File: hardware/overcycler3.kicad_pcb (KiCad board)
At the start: 2 copper layers, 208.3 x 152.4 mm, 279 parts, among them IC1 LM13700, IC2 LM13700, IC3 LM13700, P1 LPC_P1, P2 LPC_P2, P3 FT232, P4 PANEL, P5 SDCARD, P6 MIDI_IN, P7 FOOT_IN, P8 AC_IN, P9 AUDIO_OUT, Q1 BC547, SW1 RESET, U1 TLV1543, U10 MCP4922-E/P, U11 SSM2044, U12 MCP4922-E/P, U13 SSM2044, U14 MCP4922-E/P, U15 SSM2044, U16 MCP4922-E/P, U17 SSM2044, U18 MCP4922-E/P, U19 SSM2044, U2 74HC138, U20 MCP4922-E/P, U21 SSM2044, U3 LTC1660, U4 LTC1660, U5 TL074, U6 TL074, U7 LM1084IT-5.0/NOPB, U8 LM2990-5.0/NOPB, U9 LM1084IT-ADJ/NOPB

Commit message: hardware: beginning of overcycler 3 PCB
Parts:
- removed D6, D7: 1N5819, D3
- removed P3: FT232, SIL-6
- removed P4: PANEL, CONN40
- removed P5: SDCARD, SIL-7
- removed P6: MIDI_IN, SIL-2
- removed P7: FOOT_IN, SIL-2
- removed P8: AC_IN, bornier2
- removed P9: AUDIO_OUT, SIL-8
- removed R100, R105, R67, R68, R83, R85: 15k, R3-LARGE_PADS
- removed R101, R71: 6k8, R3-LARGE_PADS
- removed R102, R117, R54, R84: 820, R3-LARGE_PADS
- removed R118, R88: 390, R3-LARGE_PADS
- removed R119, R122, R50: 4k7, R3-LARGE_PADS
- removed R49, R51, R66: 22k, R3-LARGE_PADS
- removed RV2, RV3, RV4, RV5, RV6, RV7: 1k, RV2X1.5
- removed U20: MCP4922-E/P, DIP-14__300_ELL
- removed U21: SSM2044, DIP-16__300_ELL
- added C100: 470n, Capacitor_SMD:C_0805_2012Metric, F.Cu at (236.2, 123.9)
- added C101: 100u, Capacitor_Tantalum_SMD:CP_EIA-3528-21_Kemet-B, F.Cu at (247.9, 123.5)
- added C102: 22u, Capacitor_Tantalum_SMD:CP_EIA-3216-18_Kemet-A, F.Cu at (247.8, 139.9)
- added C103: 22u, Capacitor_Tantalum_SMD:CP_EIA-3216-18_Kemet-A, F.Cu at (247.8, 143.1)
- added C104: 470n, Capacitor_SMD:C_0805_2012Metric, F.Cu at (236.2, 147.3)
- added C105: 10n, Capacitor_SMD:C_1206_3216Metric, F.Cu at (242.1, 140.0)
- added C106: 10n, Capacitor_SMD:C_1206_3216Metric, F.Cu at (242.1, 143.3)
- added C107: 10n, Capacitor_SMD:C_1206_3216Metric, F.Cu at (242.1, 146.7)
- added C108: 820p, Capacitor_SMD:C_0603_1608Metric, F.Cu at (241.3, 149.6)
- added C109: 33u, Capacitor_Tantalum_SMD:CP_EIA-3216-18_Kemet-A, F.Cu at (247.8, 146.2)
- added C110: 470n, Capacitor_SMD:C_0805_2012Metric, F.Cu at (236.2, 150.3)
- added C111: 100u, Capacitor_Tantalum_SMD:CP_EIA-3528-21_Kemet-B, F.Cu at (247.9, 149.9)
- added C96: 10n, Capacitor_SMD:C_1206_3216Metric, F.Cu at (242.1, 117.0)
- added C97: 10n, Capacitor_SMD:C_1206_3216Metric, F.Cu at (242.1, 120.3)
- added C98: 820p, Capacitor_SMD:C_0603_1608Metric, F.Cu at (241.3, 123.2)
- added C99: 33u, Capacitor_Tantalum_SMD:CP_EIA-3216-18_Kemet-A, F.Cu at (247.8, 119.8)
- added FB1: FerriteBead, Inductor_SMD:L_0805_2012Metric, F.Cu at (25.4, 31.8)
- added J1: USB_B, Connector_USB:USB_B_Lumberg_2411_02_Horizontal, F.Cu at (37.2, 30.3)
- added J2: AudioJack3_Switch, Connector_Audio:Jack_6.35mm_Neutrik_NMJ6HFD2_Horizontal, F.Cu at (96.0, 37.4)
- added J3: DIN-5_180degree, DIN-5-180:DIN-5-180, F.Cu at (129.7, 29.8)
- added J4: AudioJack3_Switch, Connector_Audio:Jack_6.35mm_Neutrik_NMJ6HFD2_Horizontal, F.Cu at (169.7, 37.5)
- added J5: AudioJack3_Switch, Connector_Audio:Jack_6.35mm_Neutrik_NMJ6HFD2_Horizontal, F.Cu at (192.1, 37.5)
- added PS1: IA0505S-2W, JETEKPS:IA0505S-2W, F.Cu at (45.7, 55.9)
- added PS2: IB0503LSY-1WR1, JETEKPS:IB0503LSY, F.Cu at (38.1, 40.6)
- added R: 15k, Resistor_SMD:R_0805_2012Metric, F.Cu at (168.6, 132.7)
- added R: 15k, Resistor_SMD:R_0805_2012Metric, F.Cu at (228.2, 117.9)
- added R: 15k, Resistor_SMD:R_0805_2012Metric, F.Cu at (197.9, 135.7)
- added R: 15k, Resistor_SMD:R_0805_2012Metric, F.Cu at (168.6, 144.5)
- added R: 15k, Resistor_SMD:R_0805_2012Metric, F.Cu at (228.2, 106.1)
- added R: 15k, Resistor_SMD:R_0805_2012Metric, F.Cu at (197.9, 144.5)
- added R: 15k, Resistor_SMD:R_0805_2012Metric, F.Cu at (228.2, 129.6)
- added R: 15k, Resistor_SMD:R_0805_2012Metric, F.Cu at (228.2, 103.2)
- added R: 15k, Resistor_SMD:R_0805_2012Metric, F.Cu at (197.9, 132.7)
- added R: 15k, Resistor_SMD:R_0805_2012Metric, F.Cu at (228.2, 109.1)
- added R: 15k, Resistor_SMD:R_0805_2012Metric, F.Cu at (139.2, 144.5)
- added R: 15k, Resistor_SMD:R_0805_2012Metric, F.Cu at (228.2, 132.5)
- added R: 15k, Resistor_SMD:R_0805_2012Metric, F.Cu at (228.2, 144.3)
- added R: 15k, Resistor_SMD:R_0805_2012Metric, F.Cu at (109.8, 135.7)
- added R: 15k, Resistor_SMD:R_0805_2012Metric, F.Cu at (109.8, 132.7)
- added R: 15k, Resistor_SMD:R_0805_2012Metric, F.Cu at (168.6, 135.7)
- added R: 15k, Resistor_SMD:R_0805_2012Metric, F.Cu at (228.2, 135.5)
- added R: 15k, Resistor_SMD:R_0805_2012Metric, F.Cu at (139.2, 129.8)
- added R: 15k, Resistor_SMD:R_0805_2012Metric, F.Cu at (109.8, 144.5)
- added R: 15k, Resistor_SMD:R_0805_2012Metric, F.Cu at (197.9, 129.8)
- added R: 15k, Resistor_SMD:R_0805_2012Metric, F.Cu at (139.2, 132.7)
- added R: 15k, Resistor_SMD:R_0805_2012Metric, F.Cu at (139.2, 135.7)
- added R: 15k, Resistor_SMD:R_0805_2012Metric, F.Cu at (109.8, 129.8)
- added R: 15k, Resistor_SMD:R_0805_2012Metric, F.Cu at (168.6, 129.8)
- added R131: 820, Resistor_SMD:R_0805_2012Metric, F.Cu at (237.1, 109.1)
- added R132: 22k, Resistor_SMD:R_0805_2012Metric, F.Cu at (237.1, 112.0)
- added R133: 4k7, Resistor_SMD:R_0805_2012Metric, F.Cu at (237.1, 115.0)
- added R137: 6k8, Resistor_SMD:R_0805_2012Metric, F.Cu at (228.2, 138.4)
- added R138: 15k, Resistor_SMD:R_0805_2012Metric, F.Cu at (228.2, 141.4)
- added R140: 390, Resistor_SMD:R_0805_2012Metric, F.Cu at (232.7, 129.6)
- added R141: 820, Resistor_SMD:R_0805_2012Metric, F.Cu at (232.7, 132.5)
- added R142: 15k, Resistor_SMD:R_0805_2012Metric, F.Cu at (232.7, 135.5)
- added R143: 4k7, Resistor_SMD:R_0805_2012Metric, F.Cu at (232.7, 138.4)
- added R144: 10k, Resistor_SMD:R_0805_2012Metric, F.Cu at (232.7, 141.4)
- added R145: 470, Resistor_SMD:R_0805_2012Metric, F.Cu at (232.7, 144.3)
- added R146: 470, Resistor_SMD:R_0805_2012Metric, F.Cu at (237.1, 129.6)
- added R147: 4k7, Resistor_SMD:R_0805_2012Metric, F.Cu at (237.1, 132.5)
- added R148: 820, Resistor_SMD:R_0805_2012Metric, F.Cu at (237.1, 135.5)
- added R149: 22k, Resistor_SMD:R_0805_2012Metric, F.Cu at (237.1, 138.4)
- added R150: 4k7, Resistor_SMD:R_0805_2012Metric, F.Cu at (237.1, 141.4)
- added SW2: POWER, SPUN192600:SPUN192600, F.Cu at (53.3, 30.3)
- added Y1: 12MHz, Crystal:Crystal_SMD_HC49-SD, F.Cu at (53.3, 82.5)
- C1: value 10u -> 22p; footprint C1V5 -> Capacitor_SMD:C_0805_2012Metric
- C10, C11, C37, C38, C39, C46, C47, C8: value 10n -> 100n; footprint C2 -> Capacitor_SMD:C_0805_2012Metric
- C12, C14, C15, C16, C17, C18, C19, C20, C26, C27, C30, C6, C7, C90, C94: footprint C2 -> Capacitor_SMD:C_0805_2012Metric
- C13: value 100n -> 470u; footprint C2 -> Capacitor_Tantalum_SMD:CP_EIA-7343-43_Kemet-X
- C2, C3, C4: value 100n -> 10n; footprint C2 -> Capacitor_SMD:C_0805_2012Metric
- C21, C22: value 100n -> 10u; footprint C2 -> Capacitor_Tantalum_SMD:CP_EIA-3216-18_Kemet-A
- C23, C42: value 100u -> 100n; footprint C1.5V8V -> Capacitor_SMD:C_0805_2012Metric
- C24, C25: value 10000u 16v -> 100n; footprint Elko_vert_DM16_RM7-5_CopperClear -> Capacitor_SMD:C_0805_2012Metric
- C28, C29: value 10u -> 100n; footprint C1V5 -> Capacitor_SMD:C_0805_2012Metric
- C31: value 100p -> 10u; footprint C2 -> Capacitor_Tantalum_SMD:CP_EIA-3216-18_Kemet-A
- C32: value 100p -> 100n; footprint C2 -> Capacitor_SMD:C_0805_2012Metric
- C33: value 10u -> 100u; footprint C1V5 -> Capacitor_Tantalum_SMD:CP_EIA-3528-21_Kemet-B
- C34, C35, C43, C44: value 22u -> 100n; footprint C1V7 -> Capacitor_SMD:C_0805_2012Metric
- C36, C81: value 820p -> 100u; footprint B32520-3 -> Capacitor_Tantalum_SMD:CP_EIA-3528-21_Kemet-B
- C40, C49: value 33u -> 100n; footprint C1.5V8V -> Capacitor_SMD:C_0805_2012Metric
- C41: value 470n -> 100n; footprint C2 -> Capacitor_SMD:C_0805_2012Metric
- C45: value 820p -> 100n; footprint B32520-3 -> Capacitor_SMD:C_0805_2012Metric
- C48: value 10n -> 100u; footprint C2 -> Capacitor_Tantalum_SMD:CP_EIA-3528-21_Kemet-B
- C5: value 100u -> 10n; footprint C1.5V8V -> Capacitor_SMD:C_0805_2012Metric
- C50: value 470n -> 100p; footprint C2 -> Capacitor_SMD:C_0805_2012Metric
- C51: value 100u -> 100p; footprint C1.5V8V -> Capacitor_SMD:C_0805_2012Metric
- C52, C53, C62: footprint C1V7 -> Capacitor_Tantalum_SMD:CP_EIA-3216-18_Kemet-A
- C54: value 820p -> 470n; footprint B32520-3 -> Capacitor_SMD:C_0805_2012Metric
- C55, C56, C57, C65, C66, C75: footprint C2 -> Capacitor_SMD:C_1206_3216Metric
- C58: value 33u -> 820p; footprint C1.5V8V -> Capacitor_SMD:C_0603_1608Metric
- C59, C89: value 470n -> 33u; footprint C2 -> Capacitor_Tantalum_SMD:CP_EIA-3216-18_Kemet-A
- C60: value 100u -> 470n; footprint C1.5V8V -> Capacitor_SMD:C_0805_2012Metric
- C61, C71: value 22u -> 100u; footprint C1V7 -> Capacitor_Tantalum_SMD:CP_EIA-3528-21_Kemet-B
- C63, C72: value 820p -> 22u; footprint B32520-3 -> Capacitor_Tantalum_SMD:CP_EIA-3216-18_Kemet-A
- C64, C74, C84: value 10n -> 470n; footprint C2 -> Capacitor_SMD:C_0805_2012Metric
- C67, C76, C85: value 33u -> 10n; footprint C1.5V8V -> Capacitor_SMD:C_1206_3216Metric
- C68: value 470n -> 820p; footprint C2 -> Capacitor_SMD:C_0603_1608Metric
- C69: value 100u -> 33u; footprint C1.5V8V -> Capacitor_Tantalum_SMD:CP_EIA-3216-18_Kemet-A
- C70, C80: value 22u -> 470n; footprint C1V7 -> Capacitor_SMD:C_0805_2012Metric
- C73, C82, C83: value 10n -> 22u; footprint C2 -> Capacitor_Tantalum_SMD:CP_EIA-3216-18_Kemet-A
- C77, C86: value 470n -> 10n; footprint C2 -> Capacitor_SMD:C_1206_3216Metric
- C78: value 100u -> 820p; footprint C1.5V8V -> Capacitor_SMD:C_0603_1608Metric
- C79: value 22u -> 33u; footprint C1V7 -> Capacitor_Tantalum_SMD:CP_EIA-3216-18_Kemet-A
- C87, C95: value 100u -> 10n; footprint C1.5V8V -> Capacitor_SMD:C_1206_3216Metric
- C88: value 2u2 -> 820p; footprint C1V5 -> Capacitor_SMD:C_0603_1608Metric
- C9: value 10n -> 22p; footprint C2 -> Capacitor_SMD:C_0805_2012Metric
- C91: value 470n -> 100u; footprint C2 -> Capacitor_Tantalum_SMD:CP_EIA-3528-21_Kemet-B
- C92, C93: value 470n -> 22u; footprint C2 -> Capacitor_Tantalum_SMD:CP_EIA-3216-18_Kemet-A
- D1: value 1N5819 -> 1N4148; footprint D3 -> Diode_SMD:D_SOD-123
- D2, D3, D4, D5: footprint D3 -> Diode_SMD:D_SOD-123
- IC1, IC2, IC3: footprint DIP-16__300_ELL -> Package_SO:SO-16_3.9x9.9mm_P1.27mm
- OC1: footprint optocoupler-DIL08 -> Package_DIP:DIP-8_W7.62mm
- P1: value LPC_P1 -> FT232; footprint SIL-33 -> Connector_PinSocket_2.54mm:PinSocket_1x06_P2.54mm_Vertical
- P2: value LPC_P2 -> PANEL; footprint SIL-33 -> Connector_IDC:IDC-Header_2x20_P2.54mm_Vertical
- Q1: value BC547 -> 2SC945; footprint TO92 -> Package_TO_SOT_SMD:SOT-23
- R1: value 270 -> 1k; footprint R3-LARGE_PADS -> Resistor_SMD:R_0805_2012Metric
- R10: value 1k -> 27k; footprint R3-LARGE_PADS -> Resistor_SMD:R_0805_2012Metric
- R103: value 390 -> 6k8; footprint R3-LARGE_PADS -> Resistor_SMD:R_0805_2012Metric
- R104, R125, R44, R74: value 4k7 -> 15k; footprint R3-LARGE_PADS -> Resistor_SMD:R_0805_2012Metric
- R106: value 10k -> 390; footprint R3-LARGE_PADS -> Resistor_SMD:R_0805_2012Metric
- R107, R80: value 4k7 -> 820; footprint R3-LARGE_PADS -> Resistor_SMD:R_0805_2012Metric
- R108, R57, R87: value 820 -> 15k; footprint R3-LARGE_PADS -> Resistor_SMD:R_0805_2012Metric
- R109, R79, R96: value 22k -> 4k7; footprint R3-LARGE_PADS -> Resistor_SMD:R_0805_2012Metric
- R11: value 10k -> 1k; footprint R3-LARGE_PADS -> Resistor_SMD:R_0805_2012Metric
- R110, R59, R7: value 4k7 -> 10k; footprint R3-LARGE_PADS -> Resistor_SMD:R_0805_2012Metric
- R111, R94: value 22k -> 470; footprint R3-LARGE_PADS -> Resistor_SMD:R_0805_2012Metric
- R112, R60: value 15k -> 470; footprint R3-LARGE_PADS -> Resistor_SMD:R_0805_2012Metric
- R113, R75, R82: value 15k -> 4k7; footprint R3-LARGE_PADS -> Resistor_SMD:R_0805_2012Metric
- R114, R12, R14, R28, R53, R62, R63, R64, R65, R70, R76, R81, R86, R92: footprint R3-LARGE_PADS -> Resistor_SMD:R_0805_2012Metric
- R115, R98: value 15k -> 22k; footprint R3-LARGE_PADS -> Resistor_SMD:R_0805_2012Metric
- R116: value 6k8 -> 4k7; footprint R3-LARGE_PADS -> Resistor_SMD:R_0805_2012Metric
- R120, R52: value 15k -> 6k8; footprint R3-LARGE_PADS -> Resistor_SMD:R_0805_2012Metric
- R121, R91: value 10k -> 15k; footprint R3-LARGE_PADS -> Resistor_SMD:R_0805_2012Metric
- R123, R72: value 820 -> 390; footprint R3-LARGE_PADS -> Resistor_SMD:R_0805_2012Metric
- R124: value 22k -> 820; footprint R3-LARGE_PADS -> Resistor_SMD:R_0805_2012Metric
- R126: value 220 -> 4k7; footprint R3-LARGE_PADS -> Resistor_SMD:R_0805_2012Metric
- R127: value 120 -> 10k; footprint R3-LARGE_PADS -> Resistor_SMD:R_0805_2012Metric
- R128, R129, R61: value 10k -> 470; footprint R3-LARGE_PADS -> Resistor_SMD:R_0805_2012Metric
- R13: value 100k -> 10k; footprint R3-LARGE_PADS -> Resistor_SMD:R_0805_2012Metric
- R130: value 1k -> 4k7; footprint R3-LARGE_PADS -> Resistor_SMD:R_0805_2012Metric
- R15: value 470 -> 100k; footprint R3-LARGE_PADS -> Resistor_SMD:R_0805_2012Metric
- R16: value 3M3 -> 4k7; footprint R3-LARGE_PADS -> Resistor_SMD:R_0805_2012Metric
- R17: value 470 -> 10k; footprint R3-LARGE_PADS -> Resistor_SMD:R_0805_2012Metric
- R18, R77, R95: value 4k7 -> 470; footprint R3-LARGE_PADS -> Resistor_SMD:R_0805_2012Metric
- R19: value 100k -> 3M3; footprint R3-LARGE_PADS -> Resistor_SMD:R_0805_2012Metric
- R2: value 4k7 -> 33; footprint R3-LARGE_PADS -> Resistor_SMD:R_0805_2012Metric
- R20: value 33k -> 470; footprint R3-LARGE_PADS -> Resistor_SMD:R_0805_2012Metric
- R21: value 47k -> 270; footprint R3-LARGE_PADS -> Resistor_SMD:R_0805_2012Metric
- R22: value 150k -> 4k7; footprint R3-LARGE_PADS -> Resistor_SMD:R_0805_2012Metric
- R23: value 56k -> 4k7; footprint R3-LARGE_PADS -> Resistor_SMD:R_0805_2012Metric
- R24: value 68k -> 100k; footprint R3-LARGE_PADS -> Resistor_SMD:R_0805_2012Metric
- R25: value 68k -> 1k; footprint R3-LARGE_PADS -> Resistor_SMD:R_0805_2012Metric
- R26: value 56k -> 220; footprint R3-LARGE_PADS -> Resistor_SMD:R_0805_2012Metric
- R27: value 150k -> 33k; footprint R3-LARGE_PADS -> Resistor_SMD:R_0805_2012Metric
- R29: value 33k -> 120k; footprint R3-LARGE_PADS -> Resistor_SMD:R_0805_2012Metric
- R3: value 220 -> 10k; footprint R3-LARGE_PADS -> Resistor_SMD:R_0805_2012Metric
- R30: value 15k -> 56k; footprint R3-LARGE_PADS -> Resistor_SMD:R_0805_2012Metric
- R31: value 15k -> 82k; footprint R3-LARGE_PADS -> Resistor_SMD:R_0805_2012Metric
- R32: value 47k -> 82k; footprint R3-LARGE_PADS -> Resistor_SMD:R_0805_2012Metric
- R33: value 47k -> 56k; footprint R3-LARGE_PADS -> Resistor_SMD:R_0805_2012Metric
- R34: value 1k -> 120k; footprint R3-LARGE_PADS -> Resistor_SMD:R_0805_2012Metric
- R35: value 1k -> 47k; footprint R3-LARGE_PADS -> Resistor_SMD:R_0805_2012Metric
- R36: value 22k -> 33k; footprint R3-LARGE_PADS -> Resistor_SMD:R_0805_2012Metric
- R37, R40: value 15k -> 1k; footprint R3-LARGE_PADS -> Resistor_SMD:R_0805_2012Metric
- R38: value 15k -> 2k2; footprint R3-LARGE_PADS -> Resistor_SMD:R_0805_2012Metric
- R39: value 820 -> 2k2; footprint R3-LARGE_PADS -> Resistor_SMD:R_0805_2012Metric
- R4: value 1k -> 33; footprint R3-LARGE_PADS -> Resistor_SMD:R_0805_2012Metric
- R41: value 6k8 -> 1k; footprint R3-LARGE_PADS -> Resistor_SMD:R_0805_2012Metric
- R42, R99: value 820 -> 4k7; footprint R3-LARGE_PADS -> Resistor_SMD:R_0805_2012Metric
- R43: value 390 -> 15k; footprint R3-LARGE_PADS -> Resistor_SMD:R_0805_2012Metric
- R45: value 15k -> 47k; footprint R3-LARGE_PADS -> Resistor_SMD:R_0805_2012Metric
- R46: value 10k -> 47k; footprint R3-LARGE_PADS -> Resistor_SMD:R_0805_2012Metric
- R47: value 4k7 -> 330; footprint R3-LARGE_PADS -> Resistor_SMD:R_0805_2012Metric
- R48: value 820 -> 330; footprint R3-LARGE_PADS -> Resistor_SMD:R_0805_2012Metric
- R5: value 10k -> 1k5; footprint R3-LARGE_PADS -> Resistor_SMD:R_0805_2012Metric
- R55: value 15k -> 390; footprint R3-LARGE_PADS -> Resistor_SMD:R_0805_2012Metric
- R56: value 6k8 -> 820; footprint R3-LARGE_PADS -> Resistor_SMD:R_0805_2012Metric
- R58: value 390 -> 4k7; footprint R3-LARGE_PADS -> Resistor_SMD:R_0805_2012Metric
- R6: value 470k -> 1k; footprint R3-LARGE_PADS -> Resistor_SMD:R_0805_2012Metric
- R69: value 820 -> 6k8; footprint R3-LARGE_PADS -> Resistor_SMD:R_0805_2012Metric
- R73: value 390 -> 820; footprint R3-LARGE_PADS -> Resistor_SMD:R_0805_2012Metric
- R78: value 820 -> 470; footprint R3-LARGE_PADS -> Resistor_SMD:R_0805_2012Metric
- R8: value 1M -> 470k; footprint R3-LARGE_PADS -> Resistor_SMD:R_0805_2012Metric
- R89: value 4k7 -> 390; footprint R3-LARGE_PADS -> Resistor_SMD:R_0805_2012Metric
- R9: value 27k -> 1M; footprint R3-LARGE_PADS -> Resistor_SMD:R_0805_2012Metric
- R90, R97: value 15k -> 820; footprint R3-LARGE_PADS -> Resistor_SMD:R_0805_2012Metric
- R93: value 820 -> 10k; footprint R3-LARGE_PADS -> Resistor_SMD:R_0805_2012Metric
- RV1: value 10k -> 47k; footprint RV2X1.5 -> Potentiometer_THT:Potentiometer_Alps_RK163_Dual_Horizontal
- SW1: footprint SW_PUSH_SMALL -> Button_Switch_THT:SW_PUSH_6mm
- U1: value TLV1543 -> XT26G02ELGIGA; footprint DIP-20__300_ELL -> Package_LGA:LGA-8_8x6mm_P1.27mm
- U10, U12, U14, U16, U18: value MCP4922-E/P -> MCP4922-ESL; footprint DIP-14__300_ELL -> Package_SO:SO-14_3.9x8.65mm_P1.27mm
- U11, U13, U15, U17, U19: value SSM2044 -> SSI2144; footprint DIP-16__300_ELL -> Package_SO:SSOP-16_3.9x4.9mm_P0.635mm
- U2: value 74HC138 -> TL074; footprint DIP-16__300_ELL -> Package_SO:SO-14_3.9x8.65mm_P1.27mm
- U3: value LTC1660 -> LPC1778FBD144; footprint DIP-16__300_ELL -> Package_QFP:LQFP-144_20x20mm_P0.5mm
- U4: value LTC1660 -> TLV1543; footprint DIP-16__300_ELL -> Package_SO:SOIC-20W_7.5x12.8mm_P1.27mm
- U5: value TL074 -> 74HC138; footprint DIP-14__300_ELL -> Package_SO:SO-16_3.9x9.9mm_P1.27mm
- U6: footprint DIP-14__300_ELL -> Package_SO:SO-14_3.9x8.65mm_P1.27mm
- U7: value LM1084IT-5.0/NOPB -> AD5674R; footprint TO220_VERT_FIXED -> Package_DFN_QFN:QFN-28-1EP_4x4mm_P0.4mm_EP2.6x2.6mm; moved to F.Cu
- U8: value LM2990-5.0/NOPB -> MCP4922-ESL; footprint TO220_VERT_FIXED -> Package_SO:SO-14_3.9x8.65mm_P1.27mm; moved to F.Cu
- U9: value LM1084IT-ADJ/NOPB -> SSI2144; footprint TO220_VERT_FIXED -> Package_SO:SSOP-16_3.9x4.9mm_P0.635mm; moved to F.Cu
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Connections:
- C1 pad 1: /DAC_VREF -> /XTAL1
- C11 pad 1: GND -> +5V
- C11 pad 2: -5V -> GND
- C13 pad 1: +5V -> Net-(PS1-+Vin)
- C13 pad 2: GND -> Net-(J1-GND)
- C18 pad 1: +5V -> +3.3V
- C19 pad 1: +5V -> +3.3V
- C2 pad 1: /DAC_VREF -> +5V
- C21 pad 1: +3.3V -> +5V
- C22 pad 1: +3.3V -> GND
- C22 pad 2: GND -> -5V
- C23 pad 1: N-0000012 -> +3.3V
- C23 pad 2: NOISE -> GND
- C24 pad 1: /UNR+ -> +3.3V
- C25 pad 1: GND -> +3.3V
- C25 pad 2: /UNR- -> GND
- C26 pad 1: /UNR+ -> +3.3V
- C27 pad 1: GND -> +3.3V
- C27 pad 2: /UNR- -> GND
- C28 pad 1: +5V -> +3.3V
- C29 pad 1: GND -> +3.3V
- C29 pad 2: -5V -> GND
- C3 pad 1: /FOOT_IN -> GND
- C3 pad 2: GND -> -5V
- C30 pad 1: +5V -> +3.3V
- C31 pad 1: N-0000073 -> +3.3V
- C31 pad 2: N-0000072 -> GND
- C32 pad 1: N-0000074 -> +3.3V
- C32 pad 2: N-0000071 -> GND
- C33 pad 1: +3.3V -> GND
- C33 pad 2: GND -> Net-(Q1-B)
- C34 pad 1: N-00000160 -> +3.3V
- C34 pad 2: N-00000163 -> GND
- C35 pad 1: N-00000161 -> Net-(Q1-E)
- C35 pad 2: N-00000162 -> Net-(U2A-+)
- C36 pad 1: N-00000164 -> Net-(C36-Pad1)
- C36 pad 2: N-00000179 -> GND
- C37 pad 1: N-00000180 -> /FOOT_IN
- C37 pad 2: N-00000166 -> GND
- C38 pad 1: N-00000170 -> /P_9
- C38 pad 2: N-00000169 -> GND
- C39 pad 1: N-00000167 -> /P_8
- C39 pad 2: N-00000171 -> GND
- C4 pad 1: N-000005 -> +5V
- C4 pad 2: N-0000017 -> GND
- C40 pad 1: N-00000172 -> /P_7
- C40 pad 2: N-00000178 -> GND
- C41 pad 1: -5V -> /P_6
- C41 pad 2: N-00000174 -> GND
- C42 pad 1: /Voice #0/OUT -> /P_5
- C42 pad 2: N-00000177 -> GND
- C43 pad 1: N-00000184 -> /P_0
- C43 pad 2: N-00000187 -> GND
- C44 pad 1: N-00000185 -> /P_1
- C44 pad 2: N-00000186 -> GND
- C45 pad 1: N-00000188 -> /P_2
- C45 pad 2: N-00000203 -> GND
- C46 pad 1: N-00000204 -> /P_3
- C46 pad 2: N-00000190 -> GND
- C47 pad 1: N-00000193 -> /P_4
- C47 pad 2: N-00000192 -> GND
- C48 pad 1: N-00000191 -> Net-(C48-Pad1)
- C48 pad 2: N-00000194 -> NOISE
- C49 pad 1: N-00000196 -> Net-(U4-REF+)
- C49 pad 2: N-00000202 -> GND
- C5 pad 1: N-0000020 -> GND
- C5 pad 2: GND -> -5V
- C50 pad 1: -5V -> Net-(U6B--)
- C50 pad 2: N-00000198 -> Net-(C50-Pad2)
- C51 pad 1: /Voice #1/OUT -> Net-(U6C--)
- C51 pad 2: N-00000201 -> Net-(C51-Pad2)
- C52 pad 1: N-00000209 -> Net-(U8-VoutA)
- C53 pad 1: N-00000210 -> Net-(U8-VoutB)
- C54 pad 1: N-00000213 -> GND
- C54 pad 2: N-00000227 -> Net-(U9-FREQ_CTRL)
- C55 pad 1: N-00000228 -> Net-(U9-C1B)
- C55 pad 2: N-00000215 -> Net-(U9-C1A)
- C56 pad 1: N-00000216 -> Net-(U9-C2B)
- C56 pad 2: N-00000219 -> Net-(U9-C2A)
- C57 pad 1: N-00000208 -> Net-(U9-C3A)
- C57 pad 2: N-00000217 -> Net-(U9-C3B)
- C58 pad 1: N-00000220 -> Net-(U9-C4A)
- C58 pad 2: N-00000226 -> Net-(U9-C4B)
- C59 pad 1: -5V -> Net-(U9-OUT)
- C59 pad 2: N-00000222 -> Net-(C59-Pad2)
- C60 pad 1: /Voice #2/OUT -> -5V
- C60 pad 2: N-00000225 -> Net-(IC1A-Iabc)
- C61 pad 1: N-00000233 -> /OUT_V0
- C61 pad 2: N-00000236 -> Net-(IC1A-buffer_out)
- C62 pad 1: N-00000234 -> Net-(U10-VoutA)
- C63 pad 1: N-00000237 -> Net-(U10-VoutB)
- C63 pad 2: N-00000251 -> Net-(C63-Pad2)
- C64 pad 1: N-00000252 -> GND
- C64 pad 2: N-00000239 -> Net-(U11-FREQ_CTRL)
- C65 pad 1: N-00000240 -> Net-(U11-C1B)
- C65 pad 2: N-00000238 -> Net-(U11-C1A)
- C66 pad 1: N-00000242 -> Net-(U11-C2B)
- C66 pad 2: N-00000241 -> Net-(U11-C2A)
- C67 pad 1: N-00000244 -> Net-(U11-C3A)
- C67 pad 2: N-00000250 -> Net-(U11-C3B)
- C68 pad 1: -5V -> Net-(U11-C4A)
- C68 pad 2: N-00000246 -> Net-(U11-C4B)
- C69 pad 1: /Voice #3/OUT -> Net-(U11-OUT)
- C69 pad 2: N-00000249 -> Net-(C69-Pad2)
- C70 pad 1: N-00000257 -> -5V
- C70 pad 2: N-00000260 -> Net-(IC2B-Iabc)
- C71 pad 1: N-00000258 -> /OUT_V3
- C71 pad 2: N-00000259 -> Net-(IC2B-buffer_out)
- C72 pad 1: N-00000261 -> Net-(U12-VoutA)
- C72 pad 2: N-00000275 -> Net-(C72-Pad2)
- C73 pad 1: N-00000276 -> Net-(U12-VoutB)
- C73 pad 2: N-00000264 -> Net-(C73-Pad2)
- C74 pad 1: N-00000265 -> GND
- C74 pad 2: N-00000256 -> Net-(U13-FREQ_CTRL)
- C75 pad 1: N-00000263 -> Net-(U13-C1B)
- C75 pad 2: N-00000266 -> Net-(U13-C1A)
- C76 pad 1: N-00000268 -> Net-(U13-C2B)
- C76 pad 2: N-00000274 -> Net-(U13-C2A)
- C77 pad 1: -5V -> Net-(U13-C3A)
- C77 pad 2: N-00000270 -> Net-(U13-C3B)
- C78 pad 1: /Voice #4/OUT -> Net-(U13-C4A)
- C78 pad 2: N-00000273 -> Net-(U13-C4B)
- C79 pad 1: N-00000280 -> Net-(U13-OUT)
- C79 pad 2: N-00000283 -> Net-(C79-Pad2)
- C8 pad 1: +5V -> /RESET
- C80 pad 1: N-00000281 -> -5V
- C80 pad 2: N-00000282 -> Net-(IC1B-Iabc)
- C81 pad 1: N-00000284 -> /OUT_V1
- C81 pad 2: N-00000299 -> Net-(IC1B-buffer_out)
- C82 pad 1: N-00000300 -> Net-(U14-VoutA)
- C83 pad 1: N-00000289 -> Net-(U14-VoutB)
- C84 pad 1: N-00000287 -> GND
- C84 pad 2: N-00000290 -> Net-(U15-FREQ_CTRL)
- C85 pad 1: N-00000292 -> Net-(U15-C1B)
- C85 pad 2: N-00000298 -> Net-(U15-C1A)
- C86 pad 1: -5V -> Net-(U15-C2B)
- C86 pad 2: N-00000294 -> Net-(U15-C2A)
- C87 pad 1: /Voice #5/OUT -> Net-(U15-C3A)
- C87 pad 2: N-00000297 -> Net-(U15-C3B)
- C88 pad 1: N-0000066 -> Net-(U15-C4A)
- C88 pad 2: GND -> Net-(U15-C4B)
- C89 pad 1: GND -> Net-(U15-OUT)
- C89 pad 2: N-00000173 -> Net-(C89-Pad2)
- C9 pad 1: GND -> /XTAL2
- C9 pad 2: -5V -> GND
- C90 pad 1: GND -> -5V
- C90 pad 2: N-00000197 -> Net-(IC3A-Iabc)
- C91 pad 1: GND -> /OUT_V4
- C91 pad 2: N-00000221 -> Net-(IC3A-buffer_out)
- C92 pad 1: GND -> Net-(U16-VoutA)
- C92 pad 2: N-00000245 -> Net-(C92-Pad2)
- C93 pad 1: GND -> Net-(U16-VoutB)
- C93 pad 2: N-00000269 -> Net-(C93-Pad2)
- C94 pad 2: N-00000293 -> Net-(U17-FREQ_CTRL)
- C95 pad 1: GND -> Net-(U17-C1B)
- C95 pad 2: N-0000068 -> Net-(U17-C1A)
- D1 pad 1: N-0000062 -> Net-(D1-A)
- D1 pad 2: N-0000057 -> Net-(D1-K)
- D2 pad 1: N-0000015 -> Net-(D1-K)
- D2 pad 2: N-0000014 -> Net-(D2-K)
- D3 pad 1: N-0000014 -> Net-(D2-K)
- D3 pad 2: N-0000016 -> Net-(D3-K)
- D4 pad 1: N-0000016 -> Net-(D3-K)
- D4 pad 2: N-0000011 -> Net-(D4-K)
- D5 pad 1: N-0000011 -> Net-(D5-A)
- D5 pad 2: N-0000013 -> Net-(D5-K)
- IC1 pad 1: N-00000198 -> Net-(IC1B-Iabc)
- IC1 pad 10: N-00000176 -> Net-(IC1A-buffer_in)
- IC1 pad 12: N-00000176 -> Net-(IC1A-buffer_in)
- IC1 pad 13: N-00000175 -> Net-(IC1A--)
- IC1 pad 14: N-00000181 -> Net-(IC1A-+)
- IC1 pad 15: (no net) -> unconnected-(IC1A-bias-Pad15)
- IC1 pad 16: N-00000174 -> Net-(IC1A-Iabc)
- IC1 pad 2: (no net) -> unconnected-(IC1B-bias-Pad2)
- IC1 pad 3: N-00000205 -> Net-(IC1B-+)
- IC1 pad 4: N-00000199 -> Net-(IC1B--)
- IC1 pad 5: N-00000200 -> Net-(IC1B-buffer_in)
- IC1 pad 7: N-00000200 -> Net-(IC1B-buffer_in)
- IC1 pad 8: N-00000201 -> Net-(IC1B-buffer_out)
- IC1 pad 9: N-00000177 -> Net-(IC1A-buffer_out)
- IC2 pad 1: N-00000246 -> Net-(IC2B-Iabc)
- IC2 pad 10: N-00000224 -> Net-(IC2A-buffer_in)
- IC2 pad 12: N-00000224 -> Net-(IC2A-buffer_in)
- IC2 pad 13: N-00000223 -> Net-(IC2A--)
- IC2 pad 14: N-00000229 -> Net-(IC2A-+)
- IC2 pad 15: (no net) -> unconnected-(IC2A-bias-Pad15)
- IC2 pad 16: N-00000222 -> Net-(IC2A-Iabc)
- IC2 pad 2: (no net) -> unconnected-(IC2B-bias-Pad2)
- IC2 pad 3: N-00000253 -> Net-(IC2B-+)
- IC2 pad 4: N-00000247 -> Net-(IC2B--)
- IC2 pad 5: N-00000248 -> Net-(IC2B-buffer_in)
- IC2 pad 7: N-00000248 -> Net-(IC2B-buffer_in)
- IC2 pad 8: N-00000249 -> Net-(IC2B-buffer_out)
- IC2 pad 9: N-00000225 -> Net-(IC2A-buffer_out)
- IC3 pad 1: N-00000294 -> Net-(IC3B-Iabc)
- IC3 pad 10: N-00000272 -> Net-(IC3A-buffer_in)
- IC3 pad 12: N-00000272 -> Net-(IC3A-buffer_in)
- IC3 pad 13: N-00000271 -> Net-(IC3A--)
- IC3 pad 14: N-00000277 -> Net-(IC3A-+)
- IC3 pad 15: (no net) -> unconnected-(IC3A-bias-Pad15)
- IC3 pad 16: N-00000270 -> Net-(IC3A-Iabc)
- IC3 pad 2: (no net) -> unconnected-(IC3B-bias-Pad2)
- IC3 pad 3: N-00000301 -> Net-(IC3B-+)
- IC3 pad 5: N-00000296 -> Net-(IC3B-buffer_in)
- IC3 pad 7: N-00000296 -> Net-(IC3B-buffer_in)
- IC3 pad 8: N-00000297 -> Net-(IC3B-buffer_out)
- IC3 pad 9: N-00000273 -> Net-(IC3A-buffer_out)
- OC1 pad 2: N-0000057 -> Net-(D5-K)
- OC1 pad 3: N-0000062 -> Net-(D5-A)
- OC1 pad 7: N-0000064 -> Net-(OC1-VB)
- P1 pad 1: GND -> +3.3V
- P1 pad 2: +5V -> /PROG_TXD
- P1 pad 3: (no net) -> /PROG_RXD
- P1 pad 4: N-0000066 -> GND
- P1 pad 5: N-0000056 -> unconnected-(P1-Pad5)
- P1 pad 6: N-0000054 -> /PROG_BOOT
- P2 pad 1: +3.3V -> /LCD_DB7
- P2 pad 10: (no net) -> /LCD_RW
- P2 pad 11: N-0000060 -> /LCD_RS
- P2 pad 12: /SPI_MUX_C -> Net-(P2-P12)
- P2 pad 13: /ADC_CLK -> GND
- P2 pad 14: /ADC_EOC -> +5V
- P2 pad 15: /LCD_DB4 -> /LCD_E2
- P2 pad 16: /LCD_DB5 -> unconnected-(P2-P16-Pad16)
- P2 pad 17: /LCD_DB6 -> +3.3V
- P2 pad 18: /LCD_DB7 -> GND
- P2 pad 19: /LCD_RS -> /KP_1_R1
- P2 pad 2: (no net) -> /LCD_DB6
- P2 pad 20: /KP_8_C4 -> /KP_5_C1
- P2 pad 21: /KP_4_R4 -> /KP_2_R2
- P2 pad 22: /KP_3_R3 -> /KP_6_C2
- P2 pad 23: /KP_2_R2 -> /KP_3_R3
- P2 pad 24: /KP_1_R1 -> /KP_7_C3
- P2 pad 25: /KP_5_C1 -> /KP_4_R4
- P2 pad 26: /KP_6_C2 -> /KP_8_C4
- P2 pad 27: (no net) -> GND
- P2 pad 28: /MIDI_IN -> GND
- P2 pad 29: /KP_7_C3 -> GND
- P2 pad 3: (no net) -> /LCD_DB5
- P2 pad 30: SPI_SCK -> +3.3V
- P2 pad 31: /SPI_SSEL -> /P_9
- P2 pad 32: (no net) -> /P_0
- P2 pad 33: SPI_MOSI -> /P_8
- P2 pad 4: (no net) -> /LCD_DB4
- P2 pad 5: (no net) -> unconnected-(P2-P5-Pad5)
- P2 pad 6: (no net) -> unconnected-(P2-P6-Pad6)
- P2 pad 7: (no net) -> unconnected-(P2-P7-Pad7)
- P2 pad 8: (no net) -> unconnected-(P2-P8-Pad8)
- P2 pad 9: (no net) -> /LCD_E1
- Q1 pad 1: (no net) -> Net-(Q1-B)
- Q1 pad 2: N-0000068 -> Net-(Q1-E)
- Q1 pad 3: N-000005 -> unconnected-(Q1-C-Pad3)
- R1 pad 2: /MIDI_IN -> Net-(R1-Pad2)
- R10 pad 1: N-0000020 -> Net-(U2B-+)
- R10 pad 2: N-0000018 -> /DAC_MIXN
- R103 pad 1: N-00000269 -> /DAC_FC4
- R103 pad 2: GND -> Net-(U15-FREQ_CTRL)
- R104 pad 1: N-00000268 -> DAC_RES
- R104 pad 2: GND -> Net-(U15-Q_CTRL)
- R106 pad 1: N-00000274 -> Net-(U15-FREQ_CTRL)
- R106 pad 2: N-00000277 -> GND
- R107 pad 1: /Voice #4/DAC_VCA -> GND
- R107 pad 2: N-00000270 -> Net-(U15-SIG_IN-)
- R108 pad 1: -5V -> Net-(U15-FREQ_CTRL)
- R108 pad 2: N-00000270 -> -5V
- R109 pad 1: N-00000272 -> Net-(U15-OUT)
- R11 pad 1: GND -> Net-(C36-Pad1)
- R11 pad 2: N-000004 -> Net-(U2A--)
- R110 pad 1: N-00000273 -> Net-(C89-Pad2)
- R110 pad 2: -5V -> Net-(IC3A-+)
- R111 pad 1: NOISE -> Net-(IC3A--)
- R111 pad 2: N-00000279 -> GND
- R112 pad 1: N-00000283 -> GND
- R112 pad 2: N-00000279 -> Net-(IC3A-+)
- R113 pad 1: N-00000282 -> /DAC_VCA4
- R113 pad 2: N-00000279 -> Net-(IC3A-Iabc)
- R114 pad 1: GND -> -5V
- R114 pad 2: N-00000279 -> Net-(IC3A-Iabc)
- R115 pad 1: DAC_RES -> Net-(IC3A-buffer_in)
- R115 pad 2: N-00000285 -> GND
- R116 pad 1: /Voice #5/DAC_FC -> Net-(IC3A-buffer_out)
- R116 pad 2: N-00000293 -> -5V
- R12 pad 1: N-000003 -> GND
- R12 pad 2: N-000001 -> Net-(U2B-+)
- R120 pad 1: N-00000293 -> /DAC_FC2
- R120 pad 2: -5V -> Net-(U17-FREQ_CTRL)
- R121 pad 1: N-00000298 -> DAC_RES
- R121 pad 2: N-00000301 -> Net-(U17-Q_CTRL)
- R123 pad 1: -5V -> Net-(U17-FREQ_CTRL)
- R123 pad 2: N-00000294 -> GND
- R124 pad 1: N-00000296 -> GND
- R124 pad 2: GND -> Net-(U17-SIG_IN-)
- R125 pad 1: N-00000297 -> Net-(U17-FREQ_CTRL)
- R126 pad 1: GND -> Net-(U17-OUT)
- R126 pad 2: N-0000067 -> GND
- R127 pad 1: N-0000067 -> Net-(C99-Pad2)
- R127 pad 2: +3.3V -> Net-(IC2A-+)
- R128 pad 1: +3.3V -> Net-(IC2A--)
- R128 pad 2: N-0000066 -> GND
- R129 pad 1: N-0000068 -> GND
- R129 pad 2: -5V -> Net-(IC2A-+)
- R13 pad 1: N-0000018 -> Net-(U2B--)
- R13 pad 2: N-0000019 -> Net-(U2C--)
- R130 pad 1: +3.3V -> /DAC_VCA2
- R130 pad 2: /ADC_CLK -> Net-(IC2A-Iabc)
- R14 pad 1: N-000002 -> /FOOT_IN
- R14 pad 2: N-000001 -> Net-(J2-PadT)
- R15 pad 1: N-0000015 -> Net-(U2A--)
- R15 pad 2: N-000003 -> Net-(R15-Pad2)
- R16 pad 1: N-0000016 -> Net-(J2-PadT)
- R16 pad 2: N-0000019 -> +3.3V
- R17 pad 1: N-0000013 -> Net-(R17-Pad1)
- R17 pad 2: N-000002 -> Net-(U2C--)
- R18 pad 1: GND -> Net-(D1-A)
- R18 pad 2: N-0000021 -> Net-(U2B--)
- R19 pad 1: N-0000021 -> Net-(D2-K)
- R19 pad 2: N-0000012 -> Net-(R15-Pad2)
- R2 pad 1: GND -> /USB_DM
- R2 pad 2: N-0000064 -> Net-(J1-D-)
- R20 pad 1: N-0000075 -> Net-(D4-K)
- R20 pad 2: /Voice #4/OUT -> Net-(R17-Pad1)
- R21 pad 1: N-0000075 -> +3.3V
- R21 pad 2: /Voice #2/OUT -> /MIDI_IN
- R22 pad 1: N-0000076 -> GND
- R22 pad 2: /Voice #2/OUT -> Net-(OC1-VB)
- R23 pad 1: N-0000075 -> GND
- R23 pad 2: /Voice #0/OUT -> Net-(U2D--)
- R24 pad 1: N-0000076 -> Net-(U2D--)
- R24 pad 2: /Voice #0/OUT -> Net-(C48-Pad1)
- R25 pad 1: N-0000075 -> Net-(P2-P12)
- R25 pad 2: /Voice #1/OUT -> /LCD_CTRST
- R26 pad 1: N-0000076 -> Net-(J3-Pad4)
- R26 pad 2: /Voice #1/OUT -> Net-(D5-K)
- R27 pad 1: N-0000075 -> Net-(U6A--)
- R27 pad 2: /Voice #3/OUT -> /OUT_V4
- R28 pad 1: N-0000076 -> Net-(U6A--)
- R28 pad 2: /Voice #3/OUT -> /OUT_V2
- R29 pad 1: N-0000076 -> Net-(U6D--)
- R29 pad 2: /Voice #5/OUT -> /OUT_V2
- R3 pad 1: N-0000063 -> /RESET
- R3 pad 2: N-0000057 -> Net-(R1-Pad2)
- R30 pad 1: N-000009 -> Net-(U6A--)
- R30 pad 2: N-0000075 -> /OUT_V0
- R31 pad 1: N-0000010 -> Net-(U6D--)
- R31 pad 2: N-0000076 -> /OUT_V0
- R32 pad 1: N-0000073 -> Net-(U6A--)
- R32 pad 2: N-0000072 -> /OUT_V1
- R33 pad 1: N-0000074 -> Net-(U6D--)
- R33 pad 2: N-0000071 -> /OUT_V1
- R34 pad 1: N-0000078 -> Net-(U6A--)
- R34 pad 2: N-0000071 -> /OUT_V3
- R35 pad 1: N-0000077 -> Net-(U6D--)
- R35 pad 2: N-0000072 -> /OUT_V3
- R36 pad 1: NOISE -> Net-(U6D--)
- R36 pad 2: N-00000159 -> /OUT_V5
- R37 pad 1: N-00000163 -> +5V
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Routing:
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- removed copper zone on B.Cu, net GND
- removed copper zone on F.Cu, net GND
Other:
- board size 208.3 x 152.4 mm -> 200 x 100 mm
- board text removed: "OverCycler 2 board R6 bottom"
- board text removed: "OverCycler 2 board R6 top"

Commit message: hardware: draft PCB placement
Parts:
- moved R22 212.8 mm to (54.9, 57.0), turned to 90 degrees
- moved R26 205.6 mm to (66.4, 47.5)
- moved R21 199.0 mm to (68.6, 57.0), turned to 90 degrees
- moved R31 163.6 mm to (108.5, 60.2)
- moved R30 163.6 mm to (108.5, 57.7)
- moved C10 157.8 mm to (102.2, 110.4), turned to 90 degrees
- moved R33 149.2 mm to (127.8, 60.2), turned to 180 degrees
- moved R32 144.6 mm to (127.8, 57.7), turned to 180 degrees
- moved C11 138.6 mm to (121.3, 110.2), turned to 90 degrees
- moved C2 137.4 mm to (113.4, 73.8), turned to 180 degrees
- moved R40 132.9 mm to (146.4, 39.9), turned to -90 degrees
- moved C81 132.7 mm to (122.4, 57.7), turned to 180 degrees
- moved R44 130.9 mm to (151.4, 36.3)
- moved R37 130.9 mm to (146.4, 43.5), turned to 90 degrees
- moved R39 130.3 mm to (148.5, 39.9), turned to -90 degrees
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
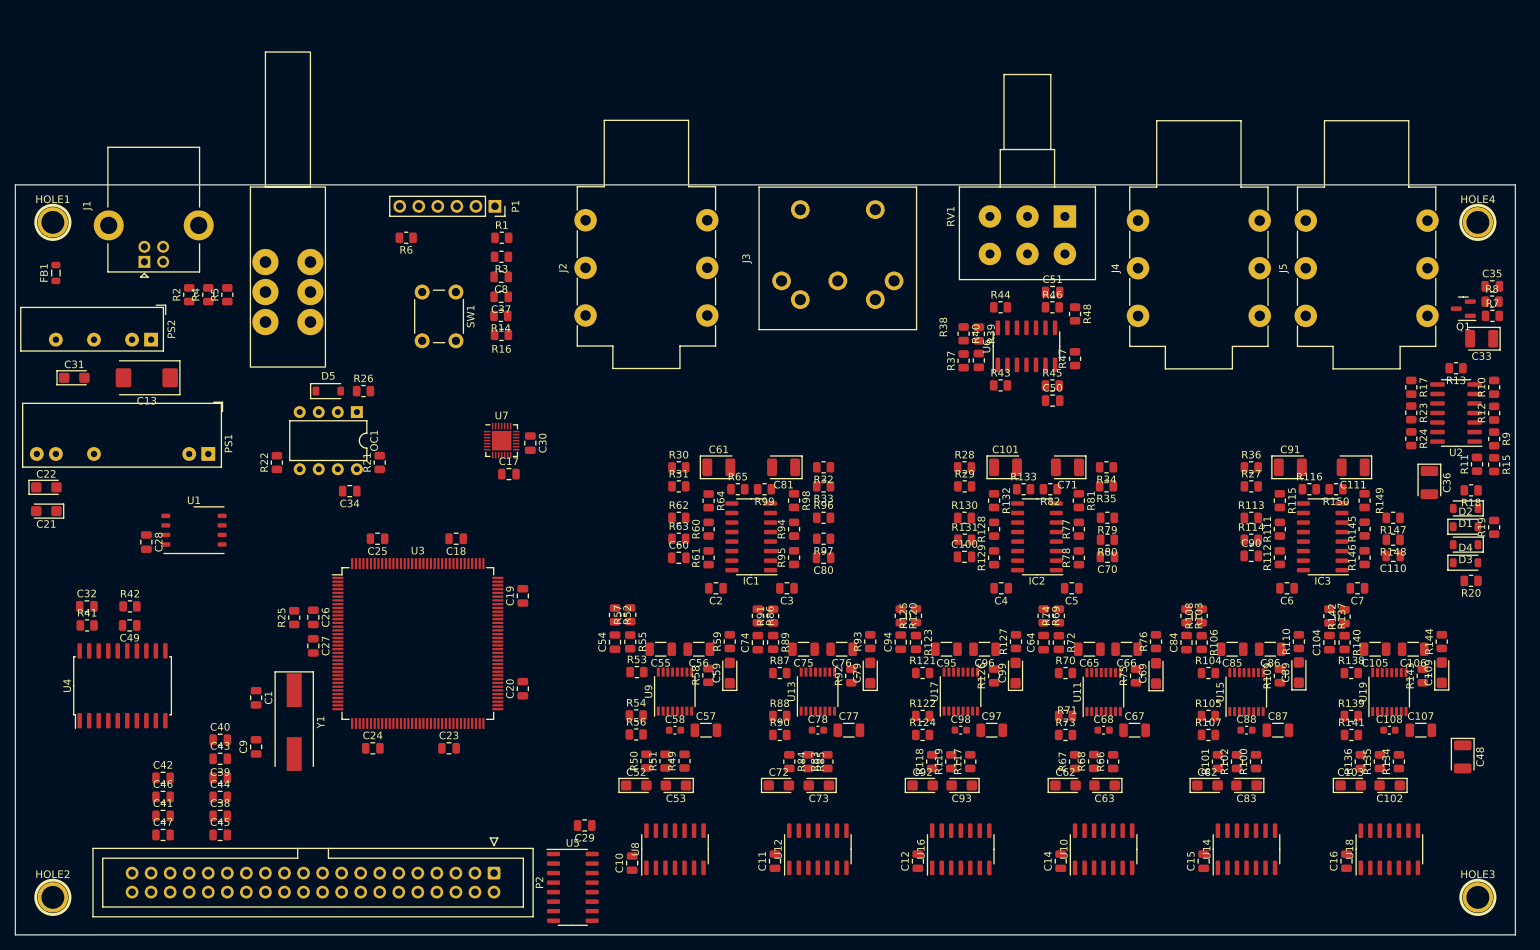
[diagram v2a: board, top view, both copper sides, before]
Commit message: hardware: CV DAC change -- misc changes -- draft routing
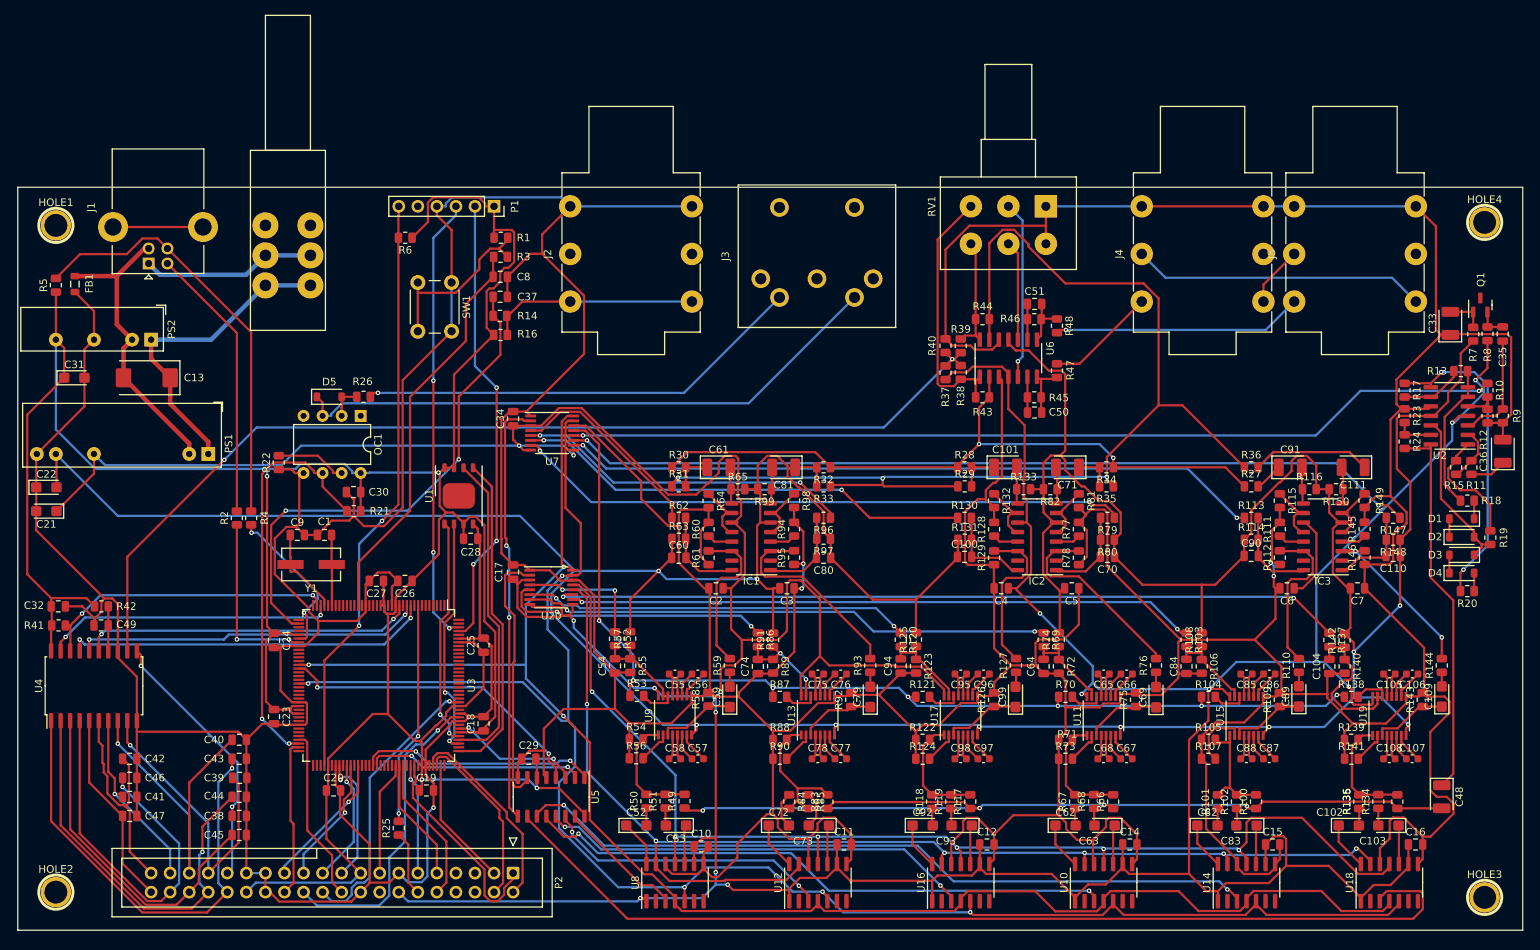
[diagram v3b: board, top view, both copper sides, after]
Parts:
- added U20: AD5328B, Package_SO:TSSOP-16_4.4x5mm_P0.65mm, F.Cu at (91.4, 73.7)
- C105, C106, C107, C55, C56, C57, C65, C66, C67, C75, C76, C77, C85, C86, C87, C95, C96, C97: footprint Capacitor_SMD:C_1206_3216Metric -> Capacitor_SMD:C_0603_1608Metric
- U7: value AD5674R -> AD5328B; footprint Package_DFN_QFN:QFN-28-1EP_4x4mm_P0.4mm_EP2.6x2.6mm -> Package_SO:TSSOP-16_4.4x5mm_P0.65mm
- Y1: footprint Crystal:Crystal_SMD_HC49-SD -> Crystal:Crystal_SMD_ECS_CSM3X-2Pin_7.6x4.1mm
- moved C28 43.2 mm to (80.7, 67.2), turned to 0 degrees
- moved U1 35.6 mm to (79.1, 61.5), turned to 90 degrees
- moved R25 31.3 mm to (71.1, 105.8)
- moved R2 30.4 mm to (49.5, 64.4)
- moved R4 30.3 mm to (51.4, 64.4)
- moved C19 28.9 mm to (74.8, 100.7), turned to 0 degrees
- moved C9 28.8 mm to (57.6, 66.7), turned to 0 degrees
- moved C20 28.6 mm to (62.4, 100.7), turned to 0 degrees
- moved C18 24.9 mm to (82.4, 91.9), turned to 90 degrees
- moved C30 24.5 mm to (65.1, 61.0), turned to 180 degrees
- moved C34 23.8 mm to (86.4, 51.2), turned to 90 degrees
- moved C23 23.7 mm to (54.5, 90.9), turned to -90 degrees
- moved C1 23.6 mm to (61.2, 66.7), turned to 180 degrees
- moved R5 22.9 mm to (25.4, 33.4)
- moved Y1 21.1 mm to (59.4, 70.6), turned to 180 degrees
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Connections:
- net Net-(J1-GND) renamed /USB_GND
- net Net-(J1-VBUS) renamed /USB_VBUS
- C13 pad 1: Net-(PS1-+Vin) -> /USB_5V
- C34 pad 1: +3.3V -> +5V
- PS1 pad 1: Net-(PS1-+Vin) -> /USB_5V
- PS2 pad 1: Net-(PS1-+Vin) -> /USB_5V
- SW2 pad 1: Net-(PS1-+Vin) -> unconnected-(SW2-A-Pad1)
- SW2 pad 3: unconnected-(SW2-C-Pad3) -> /USB_5V
- SW2 pad 4: Net-(PS1-+Vin) -> unconnected-(SW2-A-Pad4)
- SW2 pad 6: unconnected-(SW2-C-Pad6) -> /USB_5V
- U3 pad 132: /CV_SPI_SSEL -> unconnected-(U3-P1[8]-Pad132)
- U3 pad 133: /CV_SPI_MISO -> unconnected-(U3-P1[4]-Pad133)
- U3 pad 135: /CV_SPI_MOSI -> unconnected-(U3-P1[1]-Pad135)
- U3 pad 136: /CV_SPI_SCK -> unconnected-(U3-P1[0]-Pad136)
- U5 pad 7: unconnected-(U5-O7-Pad7) -> /SPI_CS7
- U5 pad 9: unconnected-(U5-O6-Pad9) -> /SPI_CS6
- U7 pad 1: /DAC_VCA0 -> GND
- U7 pad 11: DAC_MIXB -> /DAC_VCA5
- U7 pad 12: DAC_MIXA -> /DAC_MIXN
- U7 pad 13: /DAC_FC5 -> DAC_RES
- U7 pad 14: /DAC_FC4 -> GND
- U7 pad 15: GND -> SPI_MOSI
- U7 pad 16: GND -> SPI_SCK
- U7 pad 2: +5V -> /SPI_CS6
- U7 pad 3: /CV_SPI_SSEL -> +5V
- U7 pad 4: /CV_SPI_SCK -> /DAC_VCA0
- U7 pad 5: /CV_SPI_MOSI -> /DAC_VCA1
- U7 pad 6: +3.3V -> /DAC_VCA2
- U7 pad 7: DAC_RES -> /DAC_VCA3
- U7 pad 8: /DAC_MIXN -> +5V
- U7 pad 9: /DAC_VCA5 -> +5V
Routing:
- net GND: track 0.00 -> 1318.7 mm, vias 0 -> 5
- net +5V: track 0.00 -> 667.1 mm, vias 0 -> 16
- net -5V: track 0.00 -> 538.8 mm, vias 0 -> 10
- net +3.3V: track 0.00 -> 419.5 mm, vias 0 -> 4
- net SPI_MOSI: track 0.00 -> 227.7 mm, vias 0 -> 5
- net SPI_SCK: track 0.00 -> 214.7 mm, vias 0 -> 3
- net DAC_MIXA: track 0.00 -> 165.3 mm, vias 0 -> 6
- net Net-(U6D--): track 0.00 -> 160.1 mm, vias 0 -> 3
- net DAC_MIXB: track 0.00 -> 156.9 mm, vias 0 -> 6
- net DAC_RES: track 0.00 -> 141.4 mm, vias 0 -> 7
- net /ADC_MIX: track 0.00 -> 138.7 mm, vias 0 -> 2
- net /SPI_CS5: track 0.00 -> 134.5 mm
- net NOISE: track 0.00 -> 124.8 mm, vias 0 -> 4
- net /DAC_MIXN: track 0.00 -> 124.7 mm, vias 0 -> 2
- net /DAC_VCA5: track 0.00 -> 114.5 mm, vias 0 -> 2
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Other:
- board size 200 x 100 mm -> 200.7 x 99.1 mm
